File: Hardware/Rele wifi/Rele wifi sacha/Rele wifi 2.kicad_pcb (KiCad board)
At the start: 2 copper layers, 65 x 50 mm, 16 parts, among them J1 Screw_Terminal_01x02, J2 Screw_Terminal_01x03, J4 Conn_01x03_Pin, K1 G5LE-1, Q2 BC337, SW1 SW_Push, U5 PC817

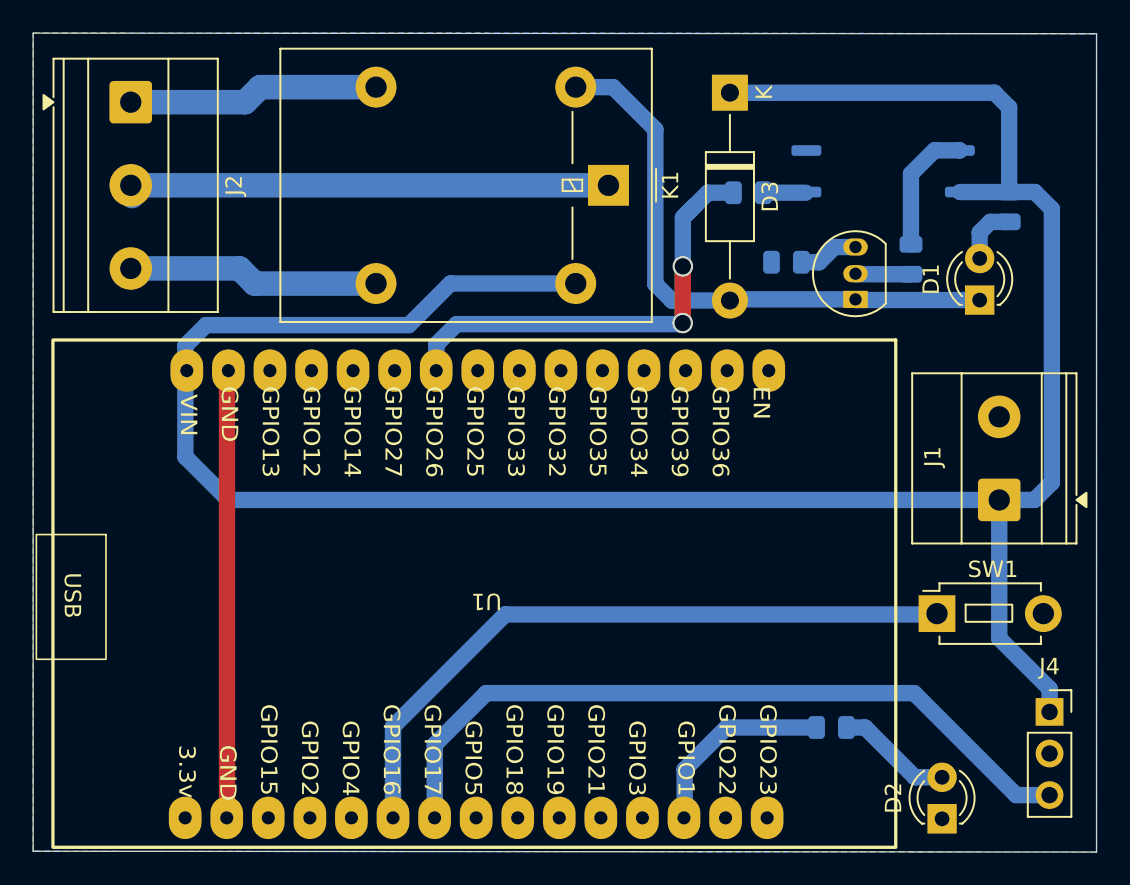
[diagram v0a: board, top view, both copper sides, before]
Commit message: actu
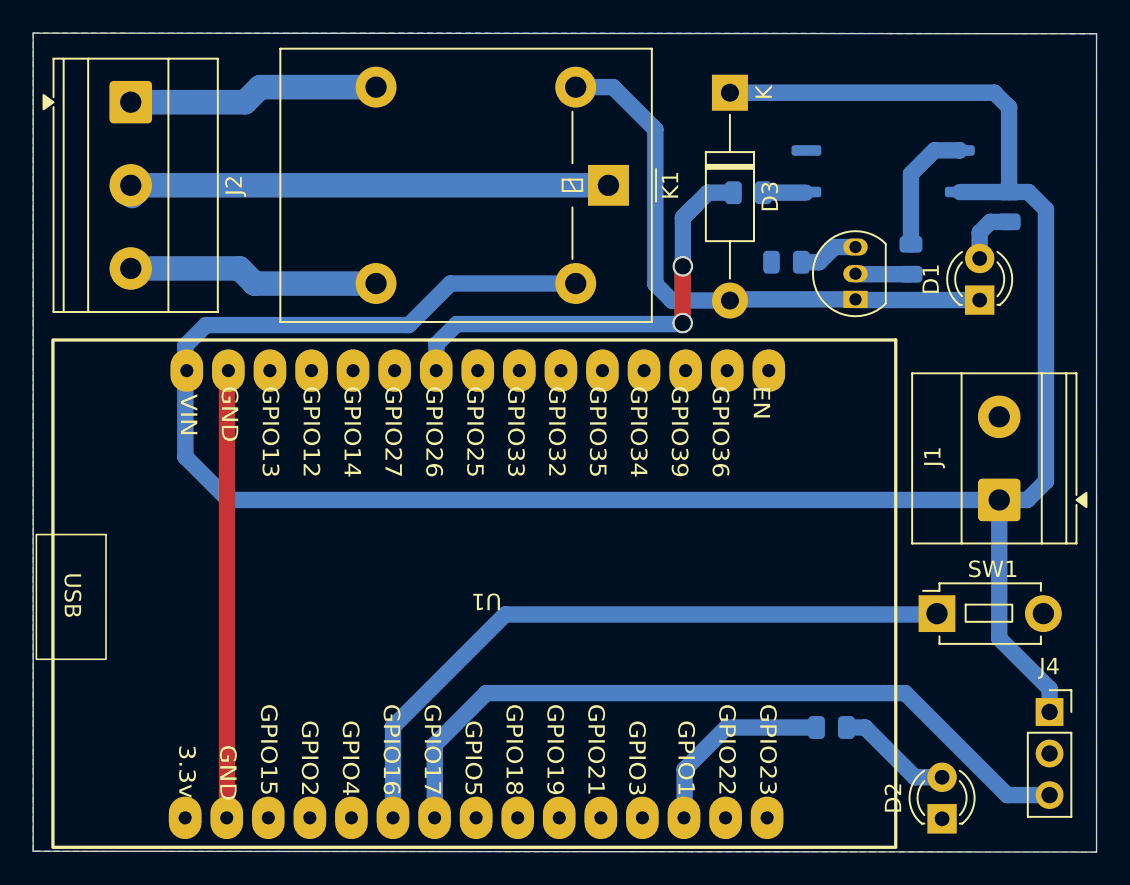
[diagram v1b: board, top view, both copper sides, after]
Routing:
- net +5V: track 146.6 -> 145.9 mm
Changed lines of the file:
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@@
+	)
+	(segment
+		(start 178.22 54.74)
+		(end 176.982277 55.977723)
+		(width 1)
+		(layer "B.Cu")
+		(net 9)
 	)
 	(segment
@@
 	)
 	(segment
+		(start 191.965 54.74)
+		(end 178.22 54.74)
+		(width 1)
+		(layer "B.Cu")
+		(net 9)
+	)
+	(segment
+		(start 192.03 54.675)
+		(end 191.965 54.74)
+		(width 1)
+		(layer "B.Cu")
+		(net 9)
+	)
+	(segment
 		(start 193.57 46.71)
 		(end 195.13 46.71)
@@
 	)
 	(segment
-		(start 191.965 54.74)
-		(end 178.22 54.74)
-		(width 1)
-		(layer "B.Cu")
-		(net 9)
-	)
-	(segment
 		(start 192.79 47.49)
 		(end 192.18 48.1)
@@
 	)
 	(segment
-		(start 192.03 54.675)
-		(end 191.965 54.74)
+		(start 192.04 48.24)
+		(end 192.04 51.21)
 		(width 1)
 		(layer "B.Cu")
@@
 	)
 	(segment
-		(start 178.22 54.74)
-		(end 176.982277 55.977723)
-		(width 1)
-		(layer "B.Cu")
-		(net 9)
-	)
-	(segment
-		(start 192.04 48.24)
-		(end 192.04 51.21)
-		(width 1)
-		(layer "B.Cu")
-		(net 9)
-	)
-	(segment
 		(start 196.955 46.71)
 		(end 199.5525 46.71)
@@
 	)
 	(segment
+		(start 214.23 64.35)
+		(end 214.23 47.74)
+		(width 1)
+		(layer "B.Cu")
+		(net 12)
+	)
+	(segment
 		(start 175.3 54.8)
 		(end 162.9 54.8)
@@
 	)
 	(segment
+		(start 213.1575 46.6675)
+		(end 211.98 46.6675)
+		(width 1)
+		(layer "B.Cu")
+		(net 12)
+	)
+	(segment
 		(start 214.45 77.02)
 		(end 211.3725 73.9425)
@@
 	)
 	(segment
-		(start 214.59 64.42)
-		(end 214.59 47.71)
+		(start 214.23 47.74)
+		(end 213.1575 46.6675)
 		(width 1)
 		(layer "B.Cu")
@@
 	)
 	(segment
-		(start 213.525 65.485)
-		(end 214.59 64.42)
+		(start 213.095 65.485)
+		(end 214.23 64.35)
 		(width 1)
 		(layer "B.Cu")
@@
 	(segment
 		(start 211.3725 65.485)
-		(end 213.525 65.485)
+		(end 213.095 65.485)
 		(width 1)
 		(layer "B.Cu")
@@
 	)
 	(segment
-		(start 213.5475 46.6675)
-		(end 211.98 46.6675)
-		(width 1)
-		(layer "B.Cu")
-		(net 12)
-	)
-	(segment
 		(start 161.642277 62.852277)
 		(end 164.275 65.485)
@@
 	)
 	(segment
-		(start 214.59 47.71)
-		(end 213.5475 46.6675)
-		(width 1)
-		(layer "B.Cu")
-		(net 12)
-	)
-	(segment
 		(start 207.88 82.43)
 		(end 206.22 82.43)
@@
 	)
 	(segment
+		(start 211.86 83.52)
+		(end 214.45 83.52)
+		(width 1)
+		(layer "B.Cu")
+		(net 37)
+	)
+	(segment
+		(start 180.03 77.29)
+		(end 205.63 77.29)
+		(width 1)
+		(layer "B.Cu")
+		(net 37)
+	)
+	(segment
 		(start 176.87 84.91)
 		(end 176.882277 84.897723)
@@
 	)
 	(segment
-		(start 206.18 77.29)
-		(end 212.41 83.52)
-		(width 1)
-		(layer "B.Cu")
-		(net 37)
-	)
-	(segment
-		(start 212.41 83.52)
-		(end 214.45 83.52)
+		(start 176.882277 84.897723)
+		(end 176.882277 80.437723)
 		(width 1)
 		(layer "B.Cu")
@@
 	)
 	(segment
-		(start 180.03 77.29)
-		(end 206.18 77.29)
-		(width 1)
-		(layer "B.Cu")
-		(net 37)
-	)
-	(segment
-		(start 176.882277 84.897723)
-		(end 176.882277 80.437723)
-		(width 1)
-		(layer "B.Cu")
+		(start 205.63 77.29)
+		(end 211.86 83.52)
+		(width 1)
+		(layer "B.Cu")
